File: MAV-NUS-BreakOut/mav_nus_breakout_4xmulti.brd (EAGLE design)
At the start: 21.4 x 39.8 mm, 148 parts

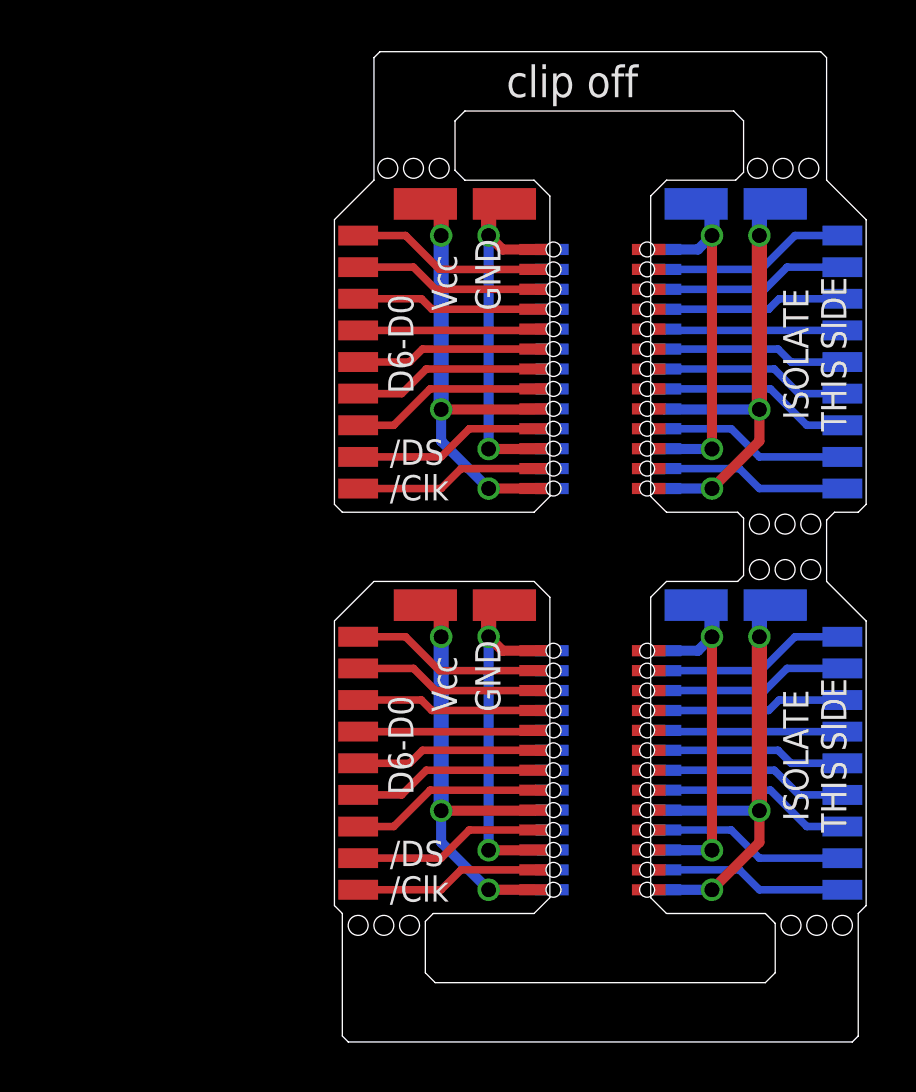
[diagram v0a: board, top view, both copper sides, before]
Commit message: update adapter PCB
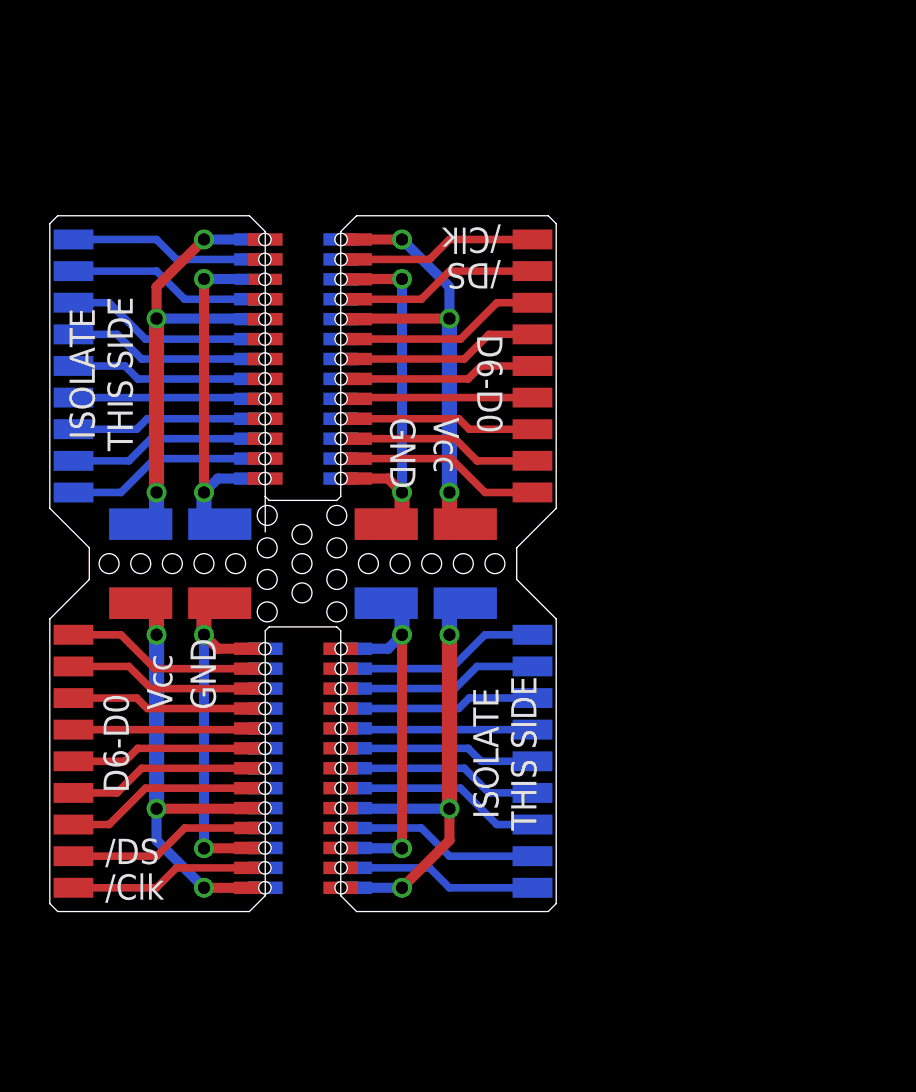
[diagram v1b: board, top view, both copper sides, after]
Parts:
- removed PAD1, PAD2, PAD7, PAD8: (no value), wirepad:SMD1,27-2,54
- removed U$1, U$10, U$106, U$107, U$108, U$109, U$11, U$110, U$117, U$12, U$121, U$122, U$123, U$124, U$125, U$126, U$127, U$128, U$129, U$13, U$130, U$131, U$132, U$133, U$134, U$135, U$136, U$137, U$138, U$139, U$140, U$2, U$23, U$24, U$25, U$26, U$27, U$28, U$29, U$3, U$30, U$31, U$32, U$33, U$34, U$35, U$4, U$5, U$6, U$7, U$8, U$9: SMD0,45, wirepad:SMD0,45-1,35
- removed U$111, U$112, U$113, U$114, U$115, U$116, U$118, U$119, U$120, U$14, U$15, U$16, U$17, U$18, U$19, U$20, U$21, U$22: SMD1, wirepad:SMD0,8-1,6
- added PAD11, PAD12, PAD13, PAD14: (no value), wirepad:SMD1,27-2,54
- added U$176, U$177, U$178, U$180, U$187, U$191, U$192, U$193, U$194, U$195, U$196, U$197, U$198, U$199, U$200, U$201, U$202, U$203, U$204, U$205, U$206, U$207, U$208, U$210, U$211, U$212, U$213, U$214, U$215, U$222, U$226, U$227, U$228, U$229, U$230, U$231, U$232, U$233, U$234, U$235, U$236, U$237, U$238, U$239, U$240, U$241, U$242, U$243, U$244, U$245: SMD0,45, wirepad:SMD0,5-1,4
- added U$179, U$209: SMD0,45, wirepad:SMD0,45-1,35
- added U$181, U$182, U$183, U$184, U$185, U$186, U$188, U$189, U$190, U$216, U$217, U$218, U$219, U$220, U$221, U$223, U$224, U$225: SMD1, wirepad:SMD0,8-1,6
- U$100, U$101, U$102, U$103, U$104, U$105, U$36, U$37, U$38, U$39, U$40, U$47, U$51, U$52, U$53, U$54, U$55, U$56, U$57, U$58, U$59, U$60, U$61, U$62, U$63, U$64, U$65, U$66, U$67, U$68, U$69, U$70, U$71, U$72, U$73, U$74, U$75, U$82, U$86, U$87, U$88, U$89, U$90, U$91, U$92, U$93, U$94, U$95, U$96, U$97, U$98, U$99: device wirepad:SMD0,45-1,35 -> wirepad:SMD0,5-1,4
- moved PAD6 13.7 mm to (2.08, 15.6), turned to 90 degrees
- moved U$93 13.1 mm to (0.25, 27.1), turned to 180 degrees
- moved PAD5 13.0 mm to (5.25, 15.6), turned to 90 degrees
- moved U$94 12.5 mm to (0.25, 17.5), turned to 180 degrees
- moved U$85 12.5 mm to (7.95, 16.9), turned to 270 degrees
- moved PAD4 12.4 mm to (2.08, 12.5)
- moved U$36 12.4 mm to (0.81, 5.83)
- moved U$37 12.4 mm to (0.81, 4.23)
- moved U$38 12.4 mm to (0.81, 1.03)
- moved U$39 12.4 mm to (0.81, 2.63)
- moved U$40 12.4 mm to (0.81, 10.6)
- moved U$47 12.4 mm to (0.81, 5.03)
- moved U$51 12.4 mm to (0.81, 3.43)
- moved U$52 12.4 mm to (0.81, 1.83)
- moved U$53 12.4 mm to (0.81, 6.63)
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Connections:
- removed net N$1: U$1.P$1, U$14.P$1
- removed net N$10: PAD1.1, U$10.P$1, U$11.P$1
- removed net N$11: PAD2.1, U$12.P$1, U$13.P$1
- removed net N$2: U$15.P$1, U$2.P$1
- removed net N$3: U$16.P$1, U$3.P$1
- removed net N$34: U$106.P$1, U$111.P$1
- removed net N$35: U$112.P$1, U$117.P$1
- removed net N$36: U$113.P$1, U$121.P$1
- removed net N$37: U$114.P$1, U$122.P$1
- removed net N$38: U$115.P$1, U$123.P$1
- removed net N$39: U$116.P$1, U$124.P$1
- removed net N$4: U$17.P$1, U$4.P$1
- removed net N$40: U$118.P$1, U$125.P$1
- removed net N$41: U$119.P$1, U$126.P$1
- removed net N$42: U$120.P$1, U$127.P$1
- removed net N$43: PAD7.1, U$107.P$1, U$108.P$1
- removed net N$44: PAD8.1, U$109.P$1, U$110.P$1
- removed net N$5: U$18.P$1, U$5.P$1
- removed net N$6: U$19.P$1, U$6.P$1
- removed net N$7: U$20.P$1, U$7.P$1
- removed net N$8: U$21.P$1, U$8.P$1
- removed net N$9: U$22.P$1, U$9.P$1
- new net N$56: U$176.P$1, U$181.P$1
- new net N$57: U$182.P$1, U$187.P$1
- new net N$58: U$183.P$1, U$191.P$1
- new net N$59: U$184.P$1, U$192.P$1
- new net N$60: U$185.P$1, U$193.P$1
- new net N$61: U$186.P$1, U$194.P$1
- new net N$62: U$188.P$1, U$195.P$1
- new net N$63: U$189.P$1, U$196.P$1
- new net N$64: U$190.P$1, U$197.P$1
- new net N$65: PAD11.1, U$177.P$1, U$178.P$1
- new net N$66: PAD12.1, U$179.P$1, U$180.P$1
- new net N$67: U$211.P$1, U$216.P$1
- new net N$68: U$217.P$1, U$222.P$1
- new net N$69: U$218.P$1, U$226.P$1
- new net N$70: U$219.P$1, U$227.P$1
- new net N$71: U$220.P$1, U$228.P$1
- new net N$72: U$221.P$1, U$229.P$1
- new net N$73: U$223.P$1, U$230.P$1
- new net N$74: U$224.P$1, U$231.P$1
- new net N$75: U$225.P$1, U$232.P$1
- new net N$76: PAD13.1, U$212.P$1, U$213.P$1
- new net N$77: PAD14.1, U$214.P$1, U$215.P$1
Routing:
- net N$76: track 0.00 -> 18.6 mm, vias 0 -> 3
- net N$65: track 0.00 -> 18.6 mm, vias 0 -> 3
- net N$43: track 18.6 -> 0.00 mm, vias 3 -> 0
- net N$10: track 18.6 -> 0.00 mm, vias 3 -> 0
- net N$44: track 14.5 -> 0.00 mm, vias 2 -> 0
- net N$66: track 0.00 -> 14.5 mm, vias 0 -> 2
- net N$11: track 14.5 -> 0.00 mm, vias 2 -> 0
- net N$77: track 0.00 -> 14.5 mm, vias 0 -> 2
- net N$35: track 7.75 -> 0.00 mm
- net N$57: track 0.00 -> 7.75 mm
- net N$68: track 0.00 -> 7.75 mm
- net N$2: track 7.75 -> 0.00 mm
- net N$9: track 7.71 -> 0.00 mm
- net N$75: track 0.00 -> 7.71 mm
- net N$64: track 0.00 -> 7.71 mm
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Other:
- board size 21.4 x 39.8 mm -> 20.3 x 27.9 mm
- board text removed: "clip off"
